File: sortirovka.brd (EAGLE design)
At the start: 173.2 x 86.7 mm, 111 parts, among them IC1 DS1307Z, IC2 MEGA8-AI, IC3 LM1117IMPX-3.3, IC4 PCF8574T, IC5 PCF8574T, IC6 PCF8574T, IC7 PCF8574T, IC8 DS1813-SMD, J1 ATTEND-MICROSD-112, U1 ADM2587EBRWZ, U2 TRACO_TEL_5-1211, X1 MKDSN1,5/3-5,08, X2 MKDSN1,5/4-5,08, X3 MKDSN1,5/4-5,08, X4 MKDSN1,5/2-5,08, X5 22-23-2021, X6 22-23-2051, X7 22-23-2041, X8 MKDSN1,5/4-5,08

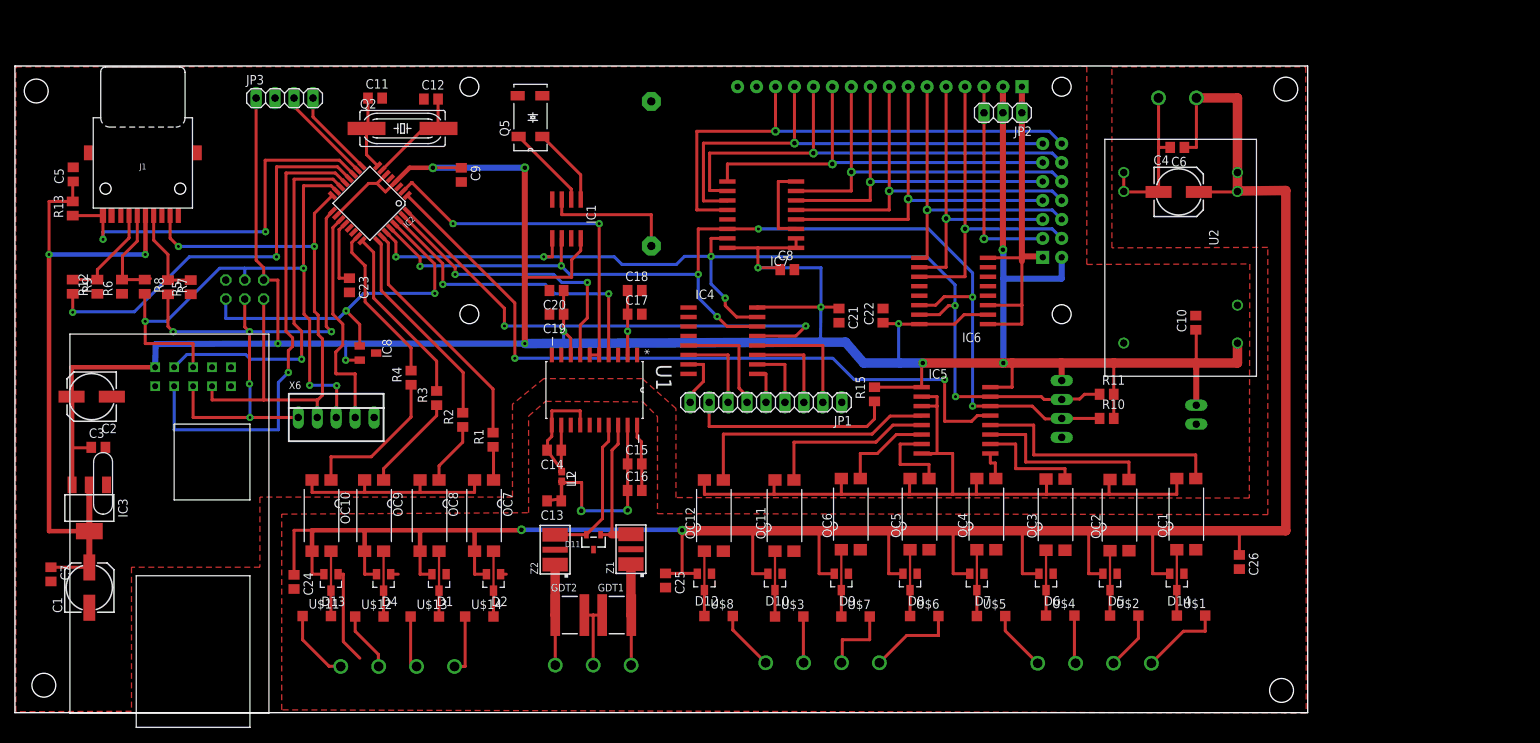
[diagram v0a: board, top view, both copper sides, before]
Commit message: Prepared to rezonver
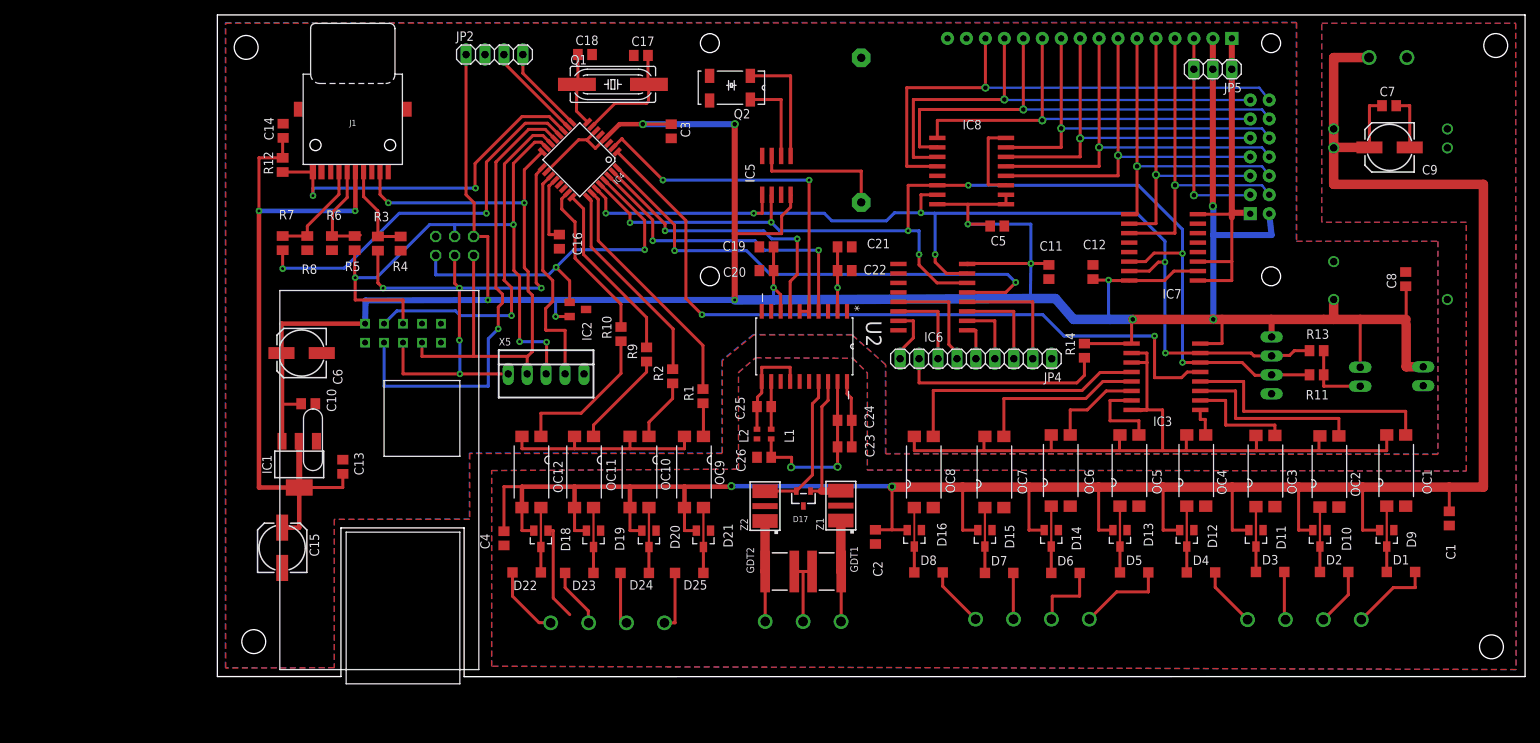
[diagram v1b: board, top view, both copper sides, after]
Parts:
- removed Q5: (no value), MyLib:MA306
- removed R15: 1k, rcl:R0805
- removed U$1, U$11, U$12, U$13, U$14, U$2, U$3, U$4, U$5, U$6, U$7, U$8: NSI45020AT1GSOD-123, MyLib:SOD123
- removed U$10: 2X16LCDBOTH, MyLib:2X16LCDBOTH
- removed U$9: W5100_MODULESMALL, MyLib:W5100_MODULE_1
- added D15, D16, D18, D19, D20, D21: BAV199, MyLib:SOT23
- added D17: CDSOT23-SM712SOT23-R, MyLib:SOT23-R
- added D22, D23, D24, D25, D3: NSI45020AT1GSOD-123, MyLib:SOD123
- added JP5: (no value), pinhead:1X03
- added LCD1: 2X16LCDBOTHM162SD07, MyLib:2X16LCDBOTH-1
- added MOD1: W5100_MODULESMALL, MyLib:W5100_MODULE_1
- added Q1: (no value), crystal:SM49
- added R14: 1k, rcl:R0805
- C1, C2, C4: value (none) -> 0.1; device rcl:153CLV-0605 -> rcl:C0805
- C11, C12: value (none) -> 0.1
- C13: value 10uF -> 0.1
- C14, C16: value 100nF -> 0.1
- C15: value 10nF -> (none); device rcl:C0805 -> rcl:153CLV-0605
- C17: value 10nF -> (none)
- C18: value 100nF -> (none)
- C19: value 100nF -> 10uF
- C20: value 10uF -> 100nF
- C21, C23, C25: value 0.1 -> 100nF
- C22, C24: value 0.1 -> 10nF
- C26: value 0.1 -> 10uF
- C6, C9: value 0.1 -> (none); device rcl:C0805 -> rcl:153CLV-0605
- D1, D2, D4, D5, D6, D7, D8: value BAV199 -> NSI45020AT1GSOD-123; device MyLib:SOT23 -> MyLib:SOD123
- D11: value CDSOT23-SM712SOT23-R -> BAV199; device MyLib:SOT23-R -> MyLib:SOT23
- IC1: value DS1307Z -> LM1117IMPX-3.3; device MyLib:SOIC8 -> lm1117:SOT223
- IC2: value MEGA8-AI -> DS1813-SMD; device atmel:TQFP32-08 -> MyLib:SOT-23
- IC3: value LM1117IMPX-3.3 -> PCF8574T; device lm1117:SOT223 -> micro-philips:SO16W
- IC4: value PCF8574T -> MEGA8-AI; device micro-philips:SO16W -> atmel:TQFP32-08
- IC5: value PCF8574T -> DS1307Z; device micro-philips:SO16W -> MyLib:SOIC8
- IC8: value DS1813-SMD -> PCF8574T; device MyLib:SOT-23 -> micro-philips:SO16W
- JP1: device pinhead:1X09 -> pinhead:2X03
- JP2: device pinhead:1X03 -> pinhead:1X04
- JP3: device pinhead:1X04 -> pinhead:1X02
- JP4: device pinhead:2X03 -> pinhead:1X09
- Q2: device crystal:SM49 -> MyLib:MA306
- R10: value 3k3 -> 50
- R12: value 3.3k -> 100k
- R13: value 100k -> 3k3; device rcl:M0805 -> rcl:R0805
- R3: value 50 -> 1.8k; device rcl:R0805 -> rcl:M0805
- R4: value 50 -> 3.3k; device rcl:R0805 -> rcl:M0805
- R5: value 3.3k -> 1.8k
- R8: value 1.8k -> 3.3k
- R9: value 1.8k -> 50; device rcl:M0805 -> rcl:R0805
- U1: value ADM2587EBRWZ -> TRACO_TEL_5-1211; device Analog Devices_By_element14_Batch_1:SOIC127P1032X265-20N -> MyLib:TRACO_POWER_TL5
- U2: value TRACO_TEL_5-1211 -> ADM2587EBRWZ; device MyLib:TRACO_POWER_TL5 -> Analog Devices_By_element14_Batch_1:SOIC127P1032X265-20N
- X1: value MKDSN1,5/3-5,08 -> MKDSN1,5/2-5,08; device MyLib:MKDSN1,5/3-5,08 -> con-phoenix-508:MKDSN1,5/2-5,08
- X2: value MKDSN1,5/4-5,08 -> 22-23-2021; device con-phoenix-508:MKDSN1,5/4-5,08 -> con-molex:22-23-2021
- X4: value MKDSN1,5/2-5,08 -> MKDSN1,5/4-5,08; device con-phoenix-508:MKDSN1,5/2-5,08 -> con-phoenix-508:MKDSN1,5/4-5,08
- X5: value 22-23-2021 -> 22-23-2051; device con-molex:22-23-2021 -> con-molex:22-23-2051
- X6: value 22-23-2051 -> 22-23-2041; device con-molex:22-23-2051 -> con-molex:22-23-2041
- X7: value 22-23-2041 -> MKDSN1,5/4-5,08; device con-molex:22-23-2041 -> con-phoenix-508:MKDSN1,5/4-5,08
- X8: value MKDSN1,5/4-5,08 -> MKDSN1,5/3-5,08; device con-phoenix-508:MKDSN1,5/4-5,08 -> MyLib:MKDSN1,5/3-5,08
- moved C7 190.0 mm to (157.3, 76.6), turned to 0 degrees
- moved C1 182.5 mm to (165.4, 21.3), turned to 270 degrees
- moved R13 167.8 mm to (147.6, 43.8), turned to 0 degrees
- moved JP3 148.9 mm to (153.4, 40.3), flipped to the bottom, turned to 270 degrees
- moved IC3 145.3 mm to (127.4, 40.3), turned to 270 degrees
- moved X1 136.2 mm to (157.2, 83.1), turned to 180 degrees
- moved D1 128.9 mm to (158.9, 14.1), turned to 0 degrees
- moved X6 125.5 mm to (141.5, 41.8), flipped to the bottom, turned to 270 degrees
- moved C9 124.5 mm to (157.4, 71.0), turned to 180 degrees
- moved C5 124.0 mm to (104.8, 60.5), turned to 0 degrees
- moved C6 120.5 mm to (11.6, 43.4)
- moved C10 119.4 mm to (12.4, 36.6), turned to 0 degrees
- moved D2 112.7 mm to (149.9, 14.1), turned to 0 degrees
- moved D4 109.5 mm to (132.1, 14.0), turned to 0 degrees
- moved U1 109.3 mm to (157.5, 62.0), flipped to the bottom
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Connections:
- removed net INT-S: IC4.4
- new net N$68: JP3.2, R11.2, R13.2
- net +24V: now also C1.1, C2.1, C4.1, C7.1, C9.+, D11.2, D15.2, D16.2, D18.2, D19.2, D20.2, D21.2, OC11.3, OC12.3, U1.+VIN@1, U1.+VIN@2, X1.1; no longer C24.1, C25.1, C26.1, C4.+, C6.1, D1.2, D2.2, D4.2, D5.2, D6.2, D7.2, D8.2, OC7.3, OC8.3, U2.+VIN@1, U2.+VIN@2, X4.1
- net +3V3: now also C13.1, C14.1, C15.+, IC1.2, IC1.TAB, R12.2; no longer C1.+, C5.1, C7.1, IC3.2, IC3.TAB, R13.2
- net +5V: now also C11.1, C12.1, C5.1, C6.+, IC1.3, IC2.2, IC3.1, IC3.16, IC4.18, IC4.4, IC4.6, IC5.8, IC8.1, IC8.16, JP1.2, JP2.1, JP5.2, LCD1.16, LCD1.2, MOD1.VCC, R14.2, U1.+VOUT, U2.2, U2.8, X2.1, X6.1; no longer C17.1, C18.1, C2.+, C9.1, IC1.8, IC2.18, IC2.4, IC2.6, IC3.3, IC4.16, IC5.1, IC5.16, IC6.2, IC7.1, JP2.2, JP4.2, R10.2, R11.2, R15.2, U$10.16, U$10.2, U$9.VCC, U1.2, U1.8, U2.+VOUT, X5.1, X7.1
- net 485_R/W: now also IC4.2, U2.5, U2.6; no longer IC2.2, U1.5, U1.6
- net A: now also D17.1, U2.18; no longer D11.1, U1.18
- net B: now also D17.2, U2.17; no longer D11.2, U1.17
- net E_RESET: now also IC4.13, MOD1.RESET; no longer IC2.13, U$9.RESET
- net E_SELECT: now also IC4.14, MOD1.SS; no longer IC2.14, U$9.SS
- net GND: now also C12.2, C13.2, C14.2, C15.-, C16.2, C17.1, C6.-, IC1.1, IC3.2, IC3.3, IC3.8, IC4.21, IC4.5, IC5.4, IC6.2, IC7.1, IC8.8, JP1.6, JP2.2, JP4.1, JP5.1, LCD1.1, LCD1.15, MOD1.GND@1, MOD1.GND@2, OC11.2, OC12.2, OC7.4, OC8.4, R4.1, R8.1, U1.-VOUT, U2.1, U2.10, U2.3, U2.9, X2.2, X5.5, X6.4; no longer C1.-, C12.1, C17.2, C2.-, C23.2, C7.2, C9.2, IC1.4, IC2.21, IC2.5, IC3.1, IC4.1, IC4.2, IC4.8, IC5.2, IC5.3, IC5.8, JP1.1, JP2.1, JP3.2, JP4.6, OC11.4, OC12.4, OC7.2, OC8.2, R12.1, R5.1, U$10.1, U$10.15, U$9.GND@1, U1.1, U1.10, U1.3, U1.9, U2.-VOUT, X5.2, X6.5, X7.4
- net GND1: now also C1.2, C2.2, C23.2, C4.2, C7.2, C9.-, D11.1, D15.1, D16.1, D17.3, D18.1, D19.1, D20.1, D21.1, OC7.2, OC8.2, U1.-VIN@1, U1.-VIN@2, U2.16, U2.20, X8.2; no longer C13.2, C15.2, C16.2, C25.2, C4.-, C6.2, D1.1, D11.3, D2.1, D4.1, D5.1, D6.1, D7.1, D8.1, OC11.2, OC12.2, U1.16, U1.20, U2.-VIN@1, U2.-VIN@2, X4.2
- net INT0: now also IC4.32, IC6.13; no longer IC2.32, IC4.13
- net INT1: now also IC3.13, IC4.1; no longer IC2.1, IC5.13
- net I_CONTRAST: now also JP5.3, LCD1.17, LCD1.3; no longer JP2.3, U$10.17, U$10.3
- net I_D0: now also IC8.4, LCD1.21, LCD1.7; no longer IC7.4, U$10.21, U$10.7
- net I_D1: now also IC8.5, LCD1.22, LCD1.8; no longer IC7.5, U$10.22, U$10.8
- net I_D2: now also IC8.6, LCD1.23, LCD1.9; no longer IC7.6, U$10.23, U$10.9
- net I_D3: now also IC8.7, LCD1.10, LCD1.24; no longer IC7.7, U$10.10, U$10.24
- net I_D4: now also IC8.9, LCD1.11, LCD1.25; no longer IC7.9, U$10.11, U$10.25
- net I_D5: now also IC8.10, LCD1.12, LCD1.26; no longer IC7.10, U$10.12, U$10.26
- net I_D6: now also IC8.11, LCD1.13, LCD1.27; no longer IC7.11, U$10.13, U$10.27
- net I_D7: now also IC8.12, LCD1.14, LCD1.28; no longer IC7.12, U$10.14, U$10.28
- net I_E: now also IC7.9, LCD1.20, LCD1.6; no longer IC6.9, U$10.20, U$10.6
- net I_RS: now also IC7.11, LCD1.18, LCD1.4; no longer IC6.11, U$10.18, U$10.4
- net I_RW: now also IC7.10, LCD1.19, LCD1.5; no longer IC6.10, U$10.19, U$10.5
- net MISO: now also IC4.16, JP1.1, MOD1.MISO, X5.2; no longer IC2.16, JP4.1, U$9.MISO, X6.2
- net MOSI: now also IC4.15, JP1.4, MOD1.MOSI, R5.2, X5.3; no longer IC2.15, JP4.4, R8.2, U$9.MOSI, X6.3
- net N$1: now also X8.1; no longer X1.1
- net N$10: now also D18.3, D22.A, OC12.4; no longer D13.3, OC10.4, U$11.A
- net N$11: now also D19.3, D23.A, OC11.4; no longer D4.3, OC9.4, U$12.A
- net N$12: now also D20.3, D24.A, OC10.4; no longer D1.3, OC8.4, U$13.A
- net N$13: now also D21.3, D25.A, OC9.4; no longer D2.3, OC7.4, U$14.A
- net N$14: now also C18.1, IC4.8, Q1.1; no longer C11.1, IC2.8, Q2.1
- net N$15: now also OC9.1; no longer OC7.1
- net N$16: now also D1.C, D9.3; no longer D14.3, U$1.C
- net N$17: now also D10.3, D2.C; no longer D5.3, U$2.C
- net N$18: now also OC10.1; no longer OC8.1
- net N$19: now also OC11.1, R9.1; no longer OC9.1, R3.1
- net N$2: now also X8.3; no longer X1.3
- net N$20: now also IC5.3; no longer IC1.3
- net N$21: now also D1.A, X4.1; no longer U$1.A, X2.1
- net N$22: now also D2.A, X4.2; no longer U$2.A, X2.2
- net N$23: now also IC5.1, Q2.1; no longer IC1.1, Q5.1
- net N$24: now also D11.3, D3.C; no longer D6.3, U$4.C
- net N$25: now also IC5.2, Q2.4; no longer IC1.2, Q5.4
- net N$26: now also C17.2, IC4.7, Q1.2; no longer C12.2, IC2.7, Q2.2
- net N$27: now also D12.3, D4.C; no longer D7.3, U$5.C
- net N$28: now also D7.A, X3.3; no longer U$3.A, X8.3
- net N$29: now also OC12.1, R10.1; no longer OC10.1, R4.1
- net N$3: now also C23.1, C24.1, C26.1, U2.19; no longer C13.1, C15.1, C16.1, U1.19
- net N$30: now also D13.3, D5.C; no longer D8.3, U$6.C
- net N$32: now also D14.3, D6.C; no longer D9.3, U$7.C
- net N$33: now also D4.A, X4.4; no longer U$5.A, X2.4
- net N$34: now also D15.3, D7.C, OC7.1; no longer D10.3, OC11.1, U$3.C
- net N$35: now also D3.A, X4.3; no longer U$4.A, X2.3
- net N$36: now also D16.3, D8.C, OC8.1; no longer D12.3, OC12.1, U$8.C
- net N$37: now also D5.A, X3.1; no longer U$6.A, X8.1
- net N$38: now also D6.A, X3.2; no longer U$7.A, X8.2
- net N$39: now also D8.A, X3.4; no longer U$8.A, X8.4
- net N$4: now also C25.2, U2.11, U2.14; no longer C14.2, U1.11, U1.14
- net N$40: now also IC3.6; no longer IC5.6
- net N$41: now also IC3.5, OC7.3; no longer IC5.5, OC11.3
- net N$42: now also IC3.4, OC8.3; no longer IC5.4, OC12.3
- net N$43: now also R7.1, R8.2; no longer R12.2, R9.1
- net N$45: now also IC6.12, JP4.2; no longer IC4.12, JP1.2
- net N$46: now also IC6.11, JP4.3; no longer IC4.11, JP1.3
- net N$47: now also IC6.10, JP4.4; no longer IC4.10, JP1.4
- net N$48: now also IC6.5, JP4.6; no longer IC4.5, JP1.6
- net N$49: now also IC6.9, JP4.5; no longer IC4.9, JP1.5
- net N$5: now also C25.1, U2.12; no longer C14.1, U1.12
- net N$50: now also IC6.7, JP4.9; no longer IC4.7, JP1.9
- net N$51: now also IC6.6, JP4.7; no longer IC4.6, JP1.7
- net N$53: now also JP4.8, R14.1; no longer JP1.8, R15.1
- net N$54: now also IC3.12; no longer IC5.12
- net N$55: now also IC3.11; no longer IC5.11
- net N$56: now also IC3.10; no longer IC5.10
- net N$57: now also IC3.9; no longer IC5.9
- net N$58: now also IC3.7; no longer IC5.7
- net N$59: now also R5.1; no longer R8.1
- net N$6: now also IC4.23, R10.2; no longer IC2.23, R4.2
- net N$60: now also R3.1, R4.2; no longer R5.2, R7.1
- net N$61: now also C16.1, IC4.20; no longer C23.1, IC2.20
- net N$62: now also D22.C, X7.1; no longer U$11.C, X3.1
- net N$63: now also D23.C, X7.2; no longer U$12.C, X3.2
- net N$64: now also IC4.10, JP2.3; no longer IC2.10, JP3.3
- net N$65: now also D24.C, X7.3; no longer U$13.C, X3.3
- net N$66: now also IC4.9, JP2.4; no longer IC2.9, JP3.4
- net N$67: now also D25.C, X7.4; no longer U$14.C, X3.4
- net N$7: now also IC4.24, R9.2; no longer IC2.24, R3.2
- net N$8: now also IC4.25; no longer IC2.25
- net N$9: now also IC4.26; no longer IC2.26
- net RESET: now also IC2.1, IC4.29, JP1.5; no longer IC2.29, IC8.1, JP4.5
- net RXD: now also IC4.30, U2.4; no longer IC2.30, U1.4
- net SCK: now also IC4.17, JP1.3, MOD1.SCK, R3.2, X5.1; no longer IC2.17, JP4.3, R7.2, U$9.SCK, X6.1
- net SCL: now also IC3.14, IC4.28, IC5.6, IC8.14, R11.1, X6.3; no longer IC1.6, IC2.28, IC4.14, IC5.14, R10.1, X7.3
- net SDA: now also IC3.15, IC4.27, IC5.5, IC8.15, R13.1, X6.2; no longer IC1.5, IC2.27, IC4.15, IC5.15, R11.1, X7.2
- net SD_DETECT: now also IC4.11, R12.1; no longer IC2.11, R13.1
- net SD_SELECT: now also IC4.12, R7.2; no longer IC2.12, R9.2
- net SPI0: now also IC4.19, X5.4; no longer IC2.19, X6.4
- net TXD: now also IC4.31, U2.7; no longer IC2.31, U1.7
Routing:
- net GND1: track 58.9 -> 38.7 mm
- net N$68: track 0.00 -> 9.65 mm
- net +24V: track 321.1 -> 329.9 mm
- net N$23: track 10.6 -> 16.1 mm
- net +3V3: track 89.8 -> 95.1 mm
- net SD_DETECT: track 52.3 -> 48.7 mm
- net N$26: track 14.2 -> 17.8 mm
- net SD_SELECT: track 55.4 -> 52.3 mm
- net E_RESET: track 63.9 -> 61.4 mm
- net N$3: track 26.7 -> 24.3 mm
- net E_SELECT: track 49.3 -> 47.0 mm
- net +5V: track 462.6 -> 460.4 mm
- net INT1: track 98.6 -> 100.4 mm
- net MOSI: track 81.9 -> 80.2 mm
- net SDA: track 142.1 -> 141.2 mm
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- added copper zone on layer 16, net GND
- added copper zone on layer 16, net GND1
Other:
- board size 173.2 x 86.7 mm -> 175.2 x 88.7 mm
